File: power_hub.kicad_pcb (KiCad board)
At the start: 2 copper layers, 61 x 59 mm, 21 parts, among them Q1 SM4185

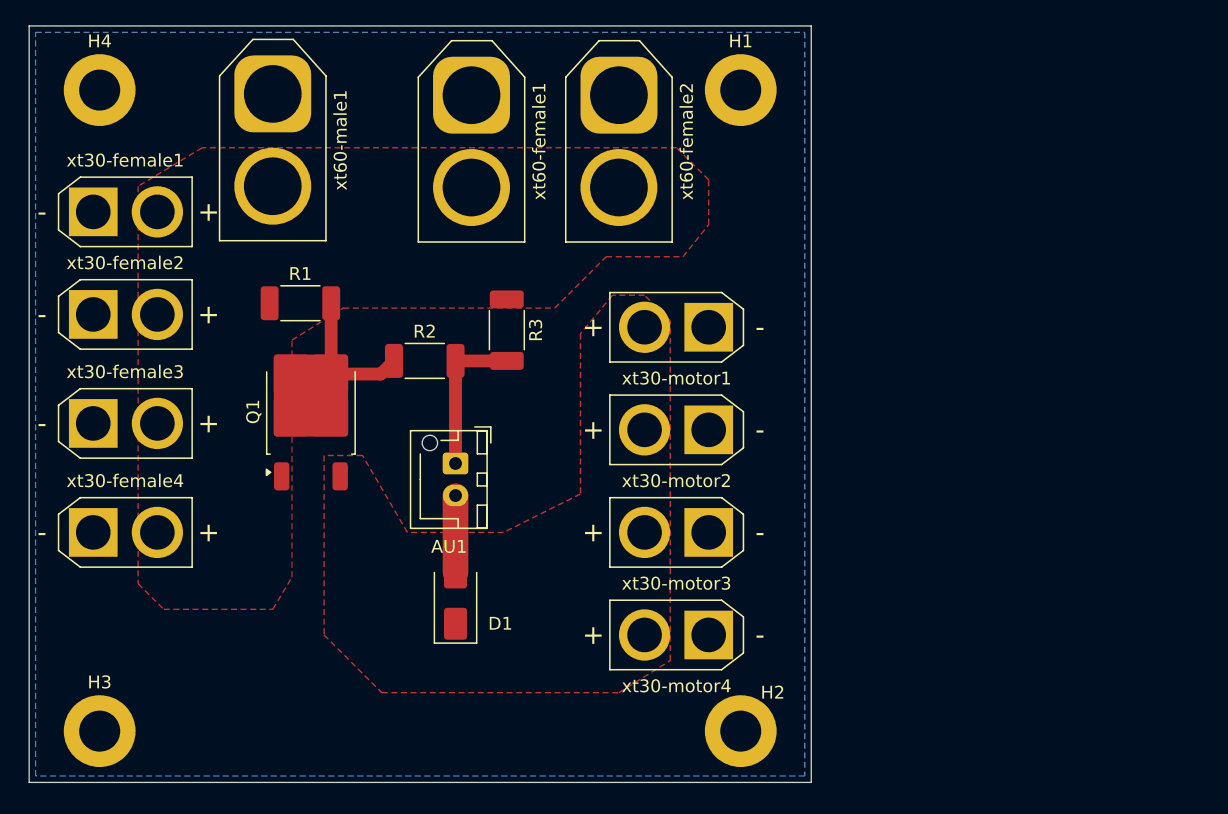
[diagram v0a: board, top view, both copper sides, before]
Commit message: v2
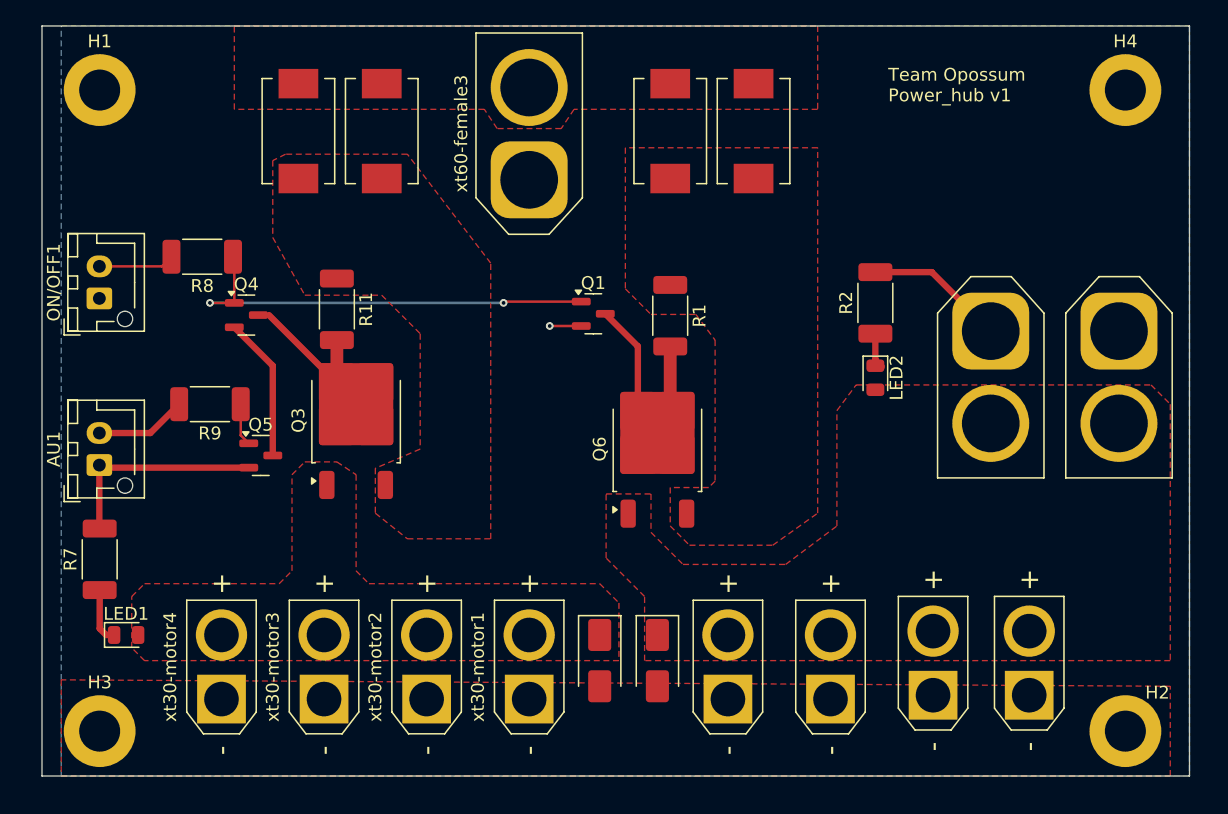
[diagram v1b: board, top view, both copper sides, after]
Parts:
- removed R3: 1K, Resistor_SMD:R_2010_5025Metric_Pad1.40x2.65mm_HandSolder
- removed xt60-male1: Conn_01x02_Pin, Connector_AMASS:AMASS_XT60-M_1x02_P7.20mm_Vertical
- added D3: D, Diode_SMD:D_SMA, F.Cu at (59.0, 64.5)
- added F1: Polyfuse, Fuse:Fuse_Bourns_MF-SM_7.98x5.44mm, F.Cu at (35.5, 23.2)
- added F2: Polyfuse, Fuse:Fuse_Bourns_MF-SM_7.98x5.44mm, F.Cu at (42.0, 23.2)
- added F3: Polyfuse, Fuse:Fuse_Bourns_MF-SM_7.98x5.44mm, F.Cu at (71.0, 23.2)
- added F4: Polyfuse, Fuse:Fuse_Bourns_MF-SM_7.98x5.44mm, F.Cu at (64.5, 23.2)
- added LED1: GREEN, LED_SMD:LED_0805_2012Metric, F.Cu at (22.1, 62.5)
- added LED2: GREEN, LED_SMD:LED_0805_2012Metric, F.Cu at (80.5, 42.4)
- added ON/OFF1: Conn_01x02_Pin, Connector_JST:JST_XH_B2B-XH-AM_1x02_P2.50mm_Vertical, F.Cu at (20.0, 36.2)
- added Q3: SM4185, Package_TO_SOT_SMD:TO-252-2, F.Cu at (40.0, 45.8)
- added Q4: 2N7002, Package_TO_SOT_SMD:SOT-23, F.Cu at (31.4, 37.5)
- added Q5: 2N7002, Package_TO_SOT_SMD:SOT-23, F.Cu at (32.6, 48.5)
- added Q6: SM4185, Package_TO_SOT_SMD:TO-252-2, F.Cu at (63.5, 48.0)
- added R11: 10k, Resistor_SMD:R_2010_5025Metric_Pad1.40x2.65mm_HandSolder, F.Cu at (38.5, 37.1)
- added R7: 5.1k, Resistor_SMD:R_2010_5025Metric_Pad1.40x2.65mm_HandSolder, F.Cu at (20.0, 56.6)
- added R8: 100R, Resistor_SMD:R_2010_5025Metric_Pad1.40x2.65mm_HandSolder, F.Cu at (28.0, 33.0)
- added R9: 100R, Resistor_SMD:R_2010_5025Metric_Pad1.40x2.65mm_HandSolder, F.Cu at (28.6, 44.5)
- added xt60-female3: Conn_01x02_Pin, Connector_AMASS:AMASS_XT60-M_1x02_P7.20mm_Vertical, F.Cu at (53.5, 27.0)
- Q1: value SM4185 -> 2N7002; footprint Package_TO_SOT_SMD:TO-252-2 -> Package_TO_SOT_SMD:SOT-23
- R2: value 100R -> 5.1k
- xt60-female1, xt60-female2: footprint Connector_AMASS:AMASS_XT60-F_1x02_P7.20mm_Vertical -> Connector_AMASS:AMASS_XT60-M_1x02_P7.20mm_Vertical
- moved H4 80.0 mm to (100.0, 20.0)
- moved xt30-female4 74.1 mm to (92.5, 67.2), turned to 90 degrees
- moved xt30-female3 68.8 mm to (85.0, 67.2), turned to 90 degrees
- moved xt30-female2 64.9 mm to (77.0, 67.5), turned to 90 degrees
- moved xt30-female1 62.4 mm to (69.0, 67.5), turned to 90 degrees
- moved H1 50.0 mm to (20.0, 20.0)
- moved xt60-female1 44.5 mm to (89.5, 38.8)
- moved xt60-female2 43.1 mm to (99.5, 38.8)
- moved xt30-motor4 38.3 mm to (29.5, 67.5), turned to 90 degrees
- moved R2 35.4 mm to (80.5, 36.6), turned to 90 degrees
- moved xt30-motor3 32.7 mm to (37.5, 67.5), turned to 90 degrees
- moved xt30-motor1 32.2 mm to (53.5, 67.5), turned to 90 degrees
- moved xt30-motor2 30.4 mm to (45.5, 67.5), turned to 90 degrees
- moved H2 30.0 mm to (100.0, 70.0)
- moved R1 28.9 mm to (64.5, 37.6), turned to -90 degrees
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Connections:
- AU1 pad 1: Net-(AU1-Pin_1) -> GND
- AU1 pad 2: GND -> Net-(AU1-Pin_2)
- D1 pad 1: 24v -> Vbat_2
- Q1 pad 1: Vbat -> ON/OFF
- Q1 pad 2: Net-(Q1-G) -> GND
- Q1 pad 3: 24v -> Net-(Q1-D)
- R1 pad 1: Vbat -> /24V_2
- R1 pad 2: Net-(Q1-G) -> Net-(Q1-D)
- R2 pad 1: Net-(Q1-G) -> Net-(LED2-K)
- R2 pad 2: Net-(AU1-Pin_1) -> GND
- xt30-female1 pad 2: Vbat -> Vbat_2
- xt30-female2 pad 2: Vbat -> Vbat_2
- xt30-female3 pad 2: Vbat -> Vbat_2
- xt30-female4 pad 2: Vbat -> Vbat_2
- xt30-motor1 pad 2: 24v -> Vbat_1
- xt30-motor2 pad 2: 24v -> Vbat_1
- xt30-motor3 pad 2: 24v -> Vbat_1
- xt30-motor4 pad 2: 24v -> Vbat_1
- xt60-female1 pad 2: Vbat -> Vbat_2
- xt60-female2 pad 2: Vbat -> Vbat_2
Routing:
- net ON/OFF: track 0.00 -> 34.7 mm, vias 0 -> 2
- net GND: track 5.95 -> 30.2 mm, vias 0 -> 1
- net Net-(Q1-D): track 0.00 -> 13.9 mm
- net Net-(AU1-Pin_1): track 12.0 -> 0.00 mm
- net Net-(Q4-S): track 0.00 -> 11.2 mm
- net Net-(Q1-G): track 10.9 -> 0.00 mm
- net Net-(Q3-G): track 0.00 -> 8.28 mm
- net Net-(AU1-Pin_2): track 0.00 -> 7.16 mm
- net Net-(ON/OFF1-Pin_2): track 0.00 -> 5.94 mm
- net Net-(LED1-K): track 0.00 -> 4.33 mm
- net AU: track 0.00 -> 3.31 mm
- net Net-(LED2-K): track 0.00 -> 2.77 mm
- net Vbat: track 0.85 -> 0.00 mm
- net Vbat_2: track 0.00 -> 0.71 mm
- net /24V_2: track 0.00 -> 0.71 mm
- added copper zone on F.Cu, net /24V_1
- added copper zone on F.Cu, net /24V_2
- added copper zone on F.Cu, net GND
- added copper zone on F.Cu, net V_IN
- added copper zone on F.Cu, net Vbat_1
- added copper zone on F.Cu, net Vbat_2
- removed copper zone on F.Cu, net 24v
- removed copper zone on F.Cu, net Vbat
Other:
- board size 61 x 59 mm -> 89.5 x 58.5 mm
- board text added: "Team Opossum Power_hub v1"

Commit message: fix issue
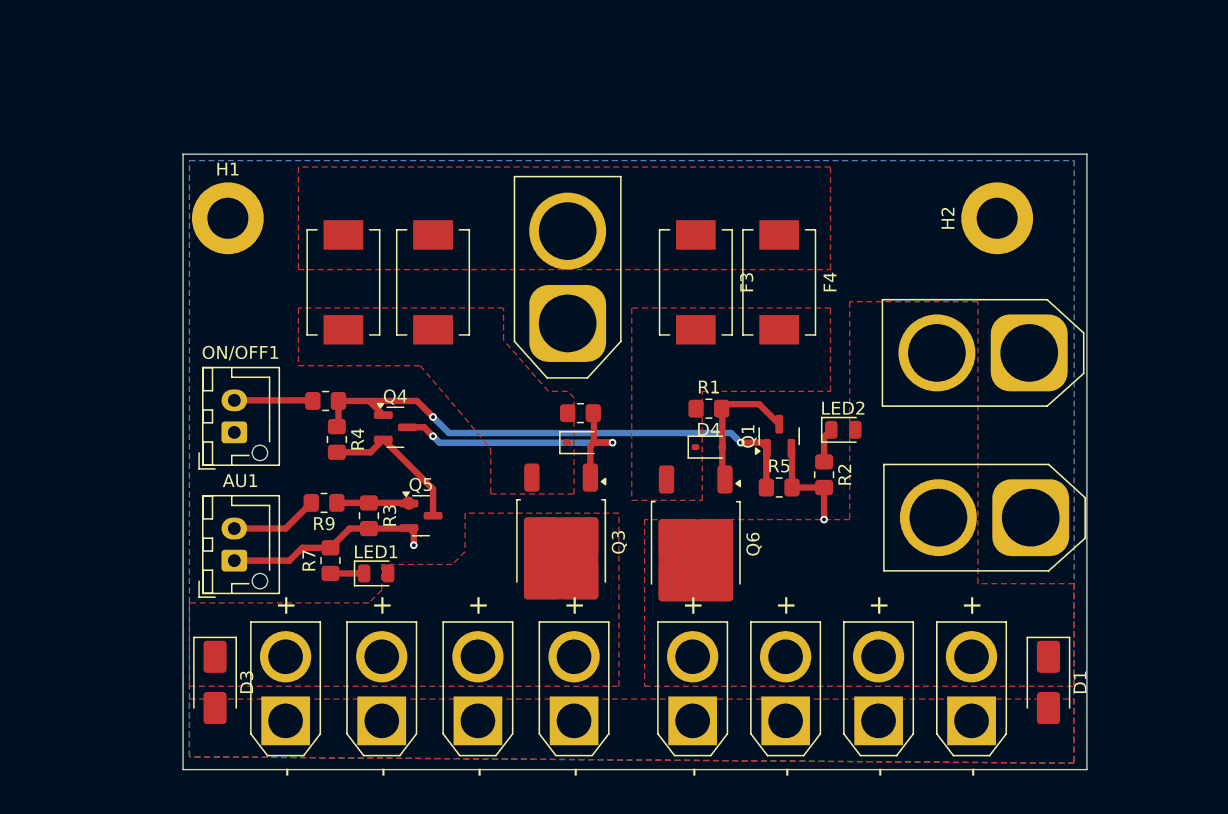
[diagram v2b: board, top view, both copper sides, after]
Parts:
- removed H3, H4: MountingHole_Pad, MountingHole:MountingHole_3.2mm_M3_DIN965_Pad
- added D2: BZT52C15S, Diode_SMD:D_SOD-323, F.Cu at (57.5, 47.5)
- added D4: BZT52C15S, Diode_SMD:D_SOD-323, F.Cu at (67.5, 47.9)
- added R3: 10k, Resistor_SMD:R_0805_2012Metric_Pad1.20x1.40mm_HandSolder, F.Cu at (41.0, 53.2)
- added R4: 10k, Resistor_SMD:R_0805_2012Metric_Pad1.20x1.40mm_HandSolder, F.Cu at (38.5, 47.2)
- added R5: 10k, Resistor_SMD:R_0805_2012Metric_Pad1.20x1.40mm_HandSolder, F.Cu at (73.0, 51.0)
- R1, R11, R2, R7, R8, R9: footprint Resistor_SMD:R_2010_5025Metric_Pad1.40x2.65mm_HandSolder -> Resistor_SMD:R_0805_2012Metric_Pad1.20x1.40mm_HandSolder
- moved H2 41.2 mm to (90.0, 30.0), turned to 90 degrees
- moved D1 30.5 mm to (94.0, 66.2)
- moved D3 30.0 mm to (29.0, 66.2)
- moved xt30-motor4 27.6 mm to (57.0, 69.2)
- moved R11 20.7 mm to (57.5, 45.2), turned to 0 degrees
- moved LED1 20.1 mm to (41.6, 57.7)
- moved xt30-motor1 19.1 mm to (34.5, 69.2)
- moved Q3 18.6 mm to (56.0, 55.3), turned to -90 degrees
- moved R7 18.0 mm to (38.0, 56.7)
- moved Q1 17.4 mm to (73.0, 47.0), turned to 90 degrees
- moved xt60-female2 16.1 mm to (92.6, 53.4), turned to 180 degrees
- moved F1 15.8 mm to (46.0, 35.0)
- moved ON/OFF1 14.8 mm to (30.5, 46.7)
- moved R8 14.8 mm to (37.6, 44.2)
- moved Q4 14.6 mm to (43.1, 46.3)
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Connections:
- Q1 pad 3: Net-(Q1-D) -> Net-(D4-A)
- Q3 pad 1: Vbat_1 -> Net-(D2-A)
- Q3 pad 2: Net-(Q3-G) -> Vbat_1
- Q4 pad 3: Net-(Q3-G) -> Net-(D2-A)
- Q6 pad 1: Vbat_2 -> Net-(D4-A)
- Q6 pad 2: Net-(Q1-D) -> Vbat_2
- R1 pad 2: Net-(Q1-D) -> Net-(D4-A)
- R11 pad 2: Net-(Q3-G) -> Net-(D2-A)
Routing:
- net Net-(D2-A): track 0.00 -> 23.1 mm, vias 0 -> 2
- net Net-(Q1-D): track 13.9 -> 0.00 mm
- net Net-(D4-A): track 0.00 -> 10.9 mm
- net Net-(Q3-G): track 8.28 -> 0.00 mm
- net ON/OFF: track 34.7 -> 41.6 mm
- net GND: track 30.2 -> 24.2 mm, vias 1 -> 2
- net AU: track 3.31 -> 5.65 mm
- net Net-(LED1-K): track 4.33 -> 2.62 mm
- net Vbat_2: track 0.71 -> 0.00 mm
- net /24V_2: track 0.71 -> 0.07 mm
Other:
- board size 89.5 x 58.5 mm -> 70.5 x 48 mm
- board text removed: "Team Opossum Power_hub v1"

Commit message: reprise v2
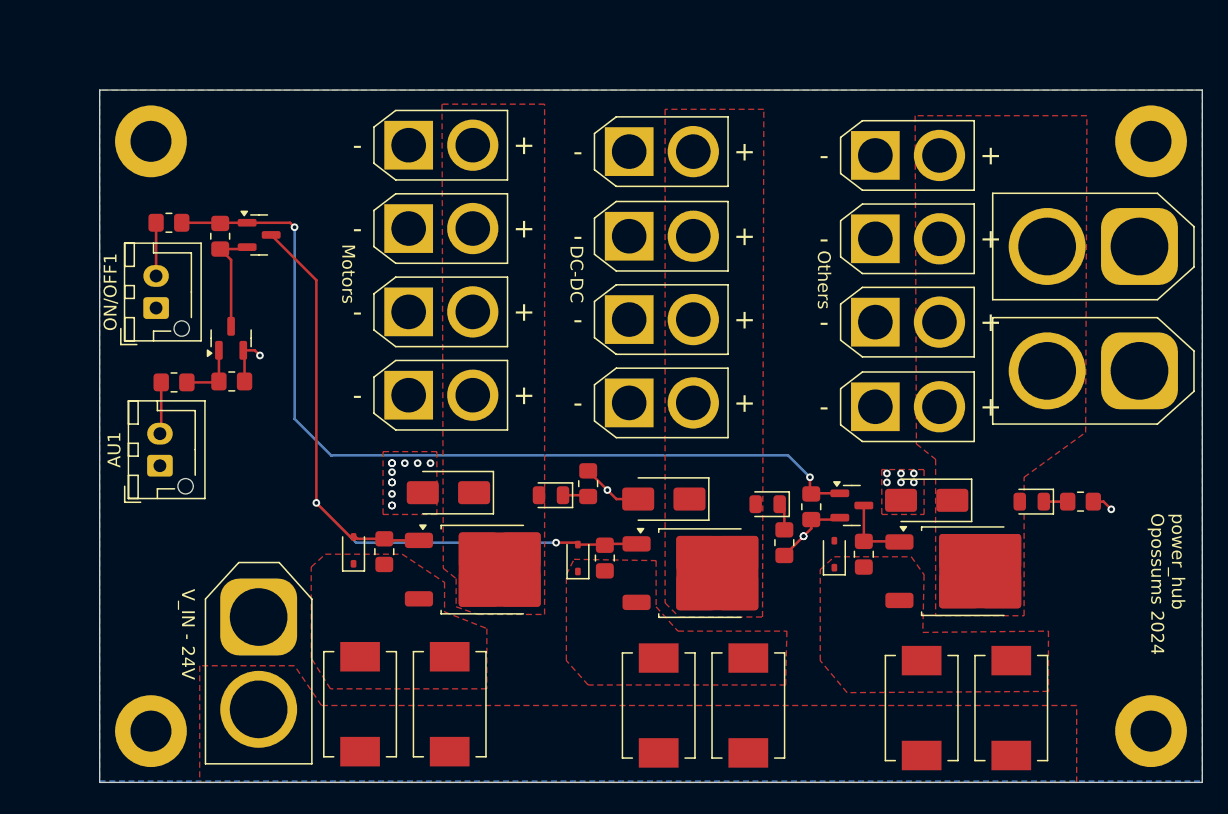
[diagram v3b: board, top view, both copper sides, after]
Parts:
- added D5: BZT52C15S, Diode_SMD:D_SOD-323, F.Cu at (57.3, 56.5)
- added D6: D, Diode_SMD:D_SMA, F.Cu at (64.0, 51.9)
- added F5: Polyfuse, Fuse:Fuse_Bourns_MF-SM_7.98x5.44mm, F.Cu at (63.6, 68.0)
- added F6: Polyfuse, Fuse:Fuse_Bourns_MF-SM_7.98x5.44mm, F.Cu at (70.6, 68.0)
- added H3: MountingHole_Pad, MountingHole:MountingHole_3.2mm_M3_DIN965_Pad, F.Cu at (102.0, 70.0)
- added H4: MountingHole_Pad, MountingHole:MountingHole_3.2mm_M3_DIN965_Pad, F.Cu at (24.0, 70.0)
- added LED3: GREEN, LED_SMD:LED_0805_2012Metric, F.Cu at (55.2, 51.6)
- added Q8: SM4185, Package_TO_SOT_SMD:TO-252-2, F.Cu at (66.9, 57.7)
- added R12: 10k, Resistor_SMD:R_0805_2012Metric_Pad1.20x1.40mm_HandSolder, F.Cu at (59.4, 56.5)
- added R13: 5.1k, Resistor_SMD:R_0805_2012Metric_Pad1.20x1.40mm_HandSolder, F.Cu at (58.1, 50.7)
- added xt30-motor5: Conn_01x02_Pin, Connector_AMASS:AMASS_XT30U-F_1x02_P5.0mm_Vertical, F.Cu at (61.3, 24.8)
- added xt30-motor6: Conn_01x02_Pin, Connector_AMASS:AMASS_XT30U-F_1x02_P5.0mm_Vertical, F.Cu at (61.3, 31.4)
- added xt30-motor7: Conn_01x02_Pin, Connector_AMASS:AMASS_XT30U-F_1x02_P5.0mm_Vertical, F.Cu at (61.3, 37.9)
- added xt30-motor8: Conn_01x02_Pin, Connector_AMASS:AMASS_XT30U-F_1x02_P5.0mm_Vertical, F.Cu at (61.3, 44.4)
- moved xt30-motor4 46.7 mm to (44.1, 24.3), turned to 0 degrees
- moved xt30-female1 46.3 mm to (80.5, 25.1), turned to 0 degrees
- moved xt30-motor3 38.8 mm to (44.1, 30.8), turned to 0 degrees
- moved F4 37.8 mm to (91.1, 68.2), turned to 90 degrees
- moved xt30-female3 37.6 mm to (80.5, 31.6), turned to 0 degrees
- moved F3 37.6 mm to (84.1, 68.2), turned to 90 degrees
- moved R7 35.4 mm to (73.4, 55.3), turned to -90 degrees
- moved F2 33.9 mm to (47.3, 67.9), turned to 90 degrees
- moved F1 33.4 mm to (40.3, 67.9), turned to 90 degrees
- moved xt60-female3 33.2 mm to (32.4, 61.1), turned to -90 degrees
- moved xt30-motor2 32.0 mm to (44.1, 37.3), turned to 0 degrees
- moved xt30-female2 31.9 mm to (80.5, 38.1), turned to 0 degrees
- moved LED1 31.0 mm to (72.1, 52.3), turned to 180 degrees
- moved xt30-motor1 27.2 mm to (44.1, 43.8), turned to 0 degrees
- moved xt30-female4 25.6 mm to (80.5, 44.7), turned to 0 degrees
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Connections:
- net /24V_2 renamed /24V_3
- net Net-(D2-A) renamed /on/off/au
- D3 pad 1: Vbat_1 -> V_moteurs
- Q3 pad 2: Vbat_1 -> V_moteurs
- xt30-motor1 pad 2: Vbat_1 -> V_moteurs
- xt30-motor2 pad 2: Vbat_1 -> V_moteurs
- xt30-motor3 pad 2: Vbat_1 -> V_moteurs
- xt30-motor4 pad 2: Vbat_1 -> V_moteurs
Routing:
- net /on/off/au: track 23.1 -> 58.0 mm
- net ON/OFF: track 41.6 -> 69.6 mm
- net GND: track 24.2 -> 16.3 mm, vias 2 -> 22
- net Net-(D4-A): track 10.9 -> 5.59 mm
- net Net-(Q4-S): track 11.6 -> 8.54 mm
- net Net-(AU1-Pin_2): track 6.83 -> 4.04 mm
- net Net-(LED3-K): track 0.00 -> 2.00 mm
- net Net-(ON/OFF1-Pin_2): track 6.15 -> 4.15 mm
- net Net-(LED2-K): track 2.73 -> 1.86 mm
- net AU: track 5.65 -> 4.96 mm
- added copper zone on F.Cu, net /24V_2
- added copper zone on F.Cu, net V_moteurs
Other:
- board size 70.5 x 48 mm -> 86 x 54 mm
- board text added: "DC-DC"
- board text added: "Motors"
- board text added: "Others"
- board text added: "V_IN - 24V"
- board text added: "power_hub Opossums 2024"
